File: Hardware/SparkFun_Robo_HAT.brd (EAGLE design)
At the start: 64.9 x 56.1 mm, 227 parts, among them J1 RASPBERRYPI-40-PIN-GPIO_PTH_R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, J11 EXT MTR PWR, J18 ISP, J2 CORTEX_DEBUGPTH, J20 USB C, J7 EXT SERVO PWR, J8 EXT 5V PWR, Q1 310mA/60V/1.6Ω, Q23 20V/0.2A/8MHz/1.2Ω/1Vth, Q24 20V/0.2A/8MHz/1.2Ω/1Vth, Q27 20V/0.2A/8MHz/1.2Ω/1Vth, Q28 20V/0.2A/8MHz/1.2Ω/1Vth, Q4 310mA/60V/1.6Ω, Q5 20V/4.2A/52mΩ/1.4W, Q7 20V/4.2A/52mΩ/1.4W, Q9 20V/4.2A/52mΩ/1.4W, U1 PCA9685, U4 ATTINY84-ARDUINO, U5 DRV8835, U6 CY8C4245LQI-483, U7 9DoF IMU, U8 1.8V/100mA

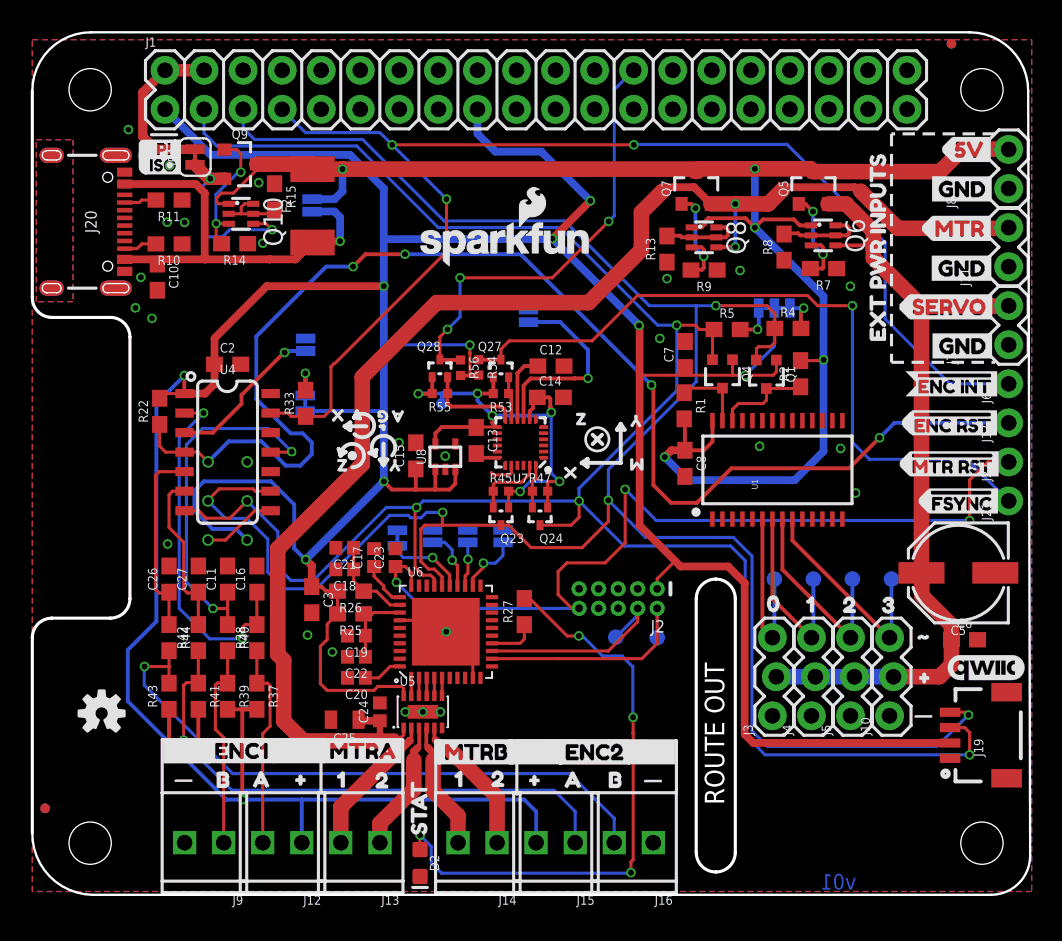
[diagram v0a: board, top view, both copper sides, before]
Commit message: sch cleanup and drc stuff in brd
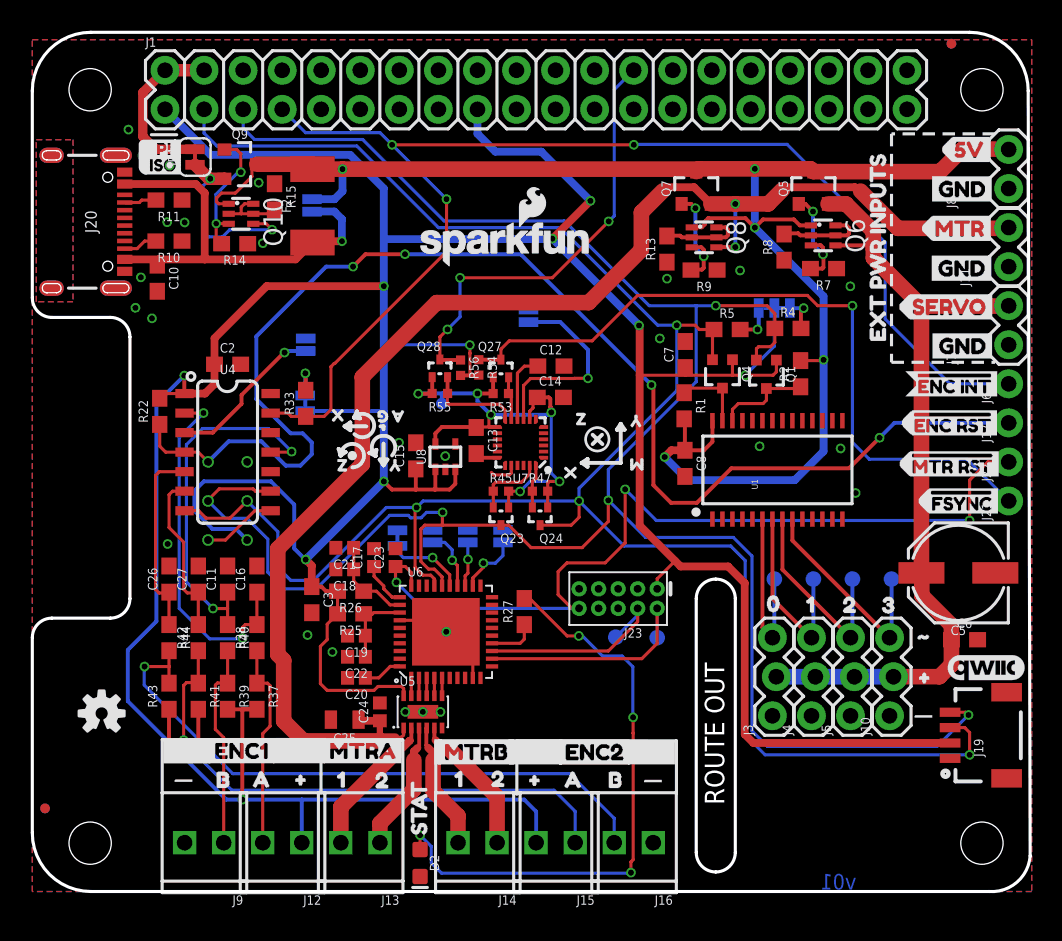
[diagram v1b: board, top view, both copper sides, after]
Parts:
- removed J2: CORTEX_DEBUGPTH, Pete_Connectors_Retired:2X5-PTH-1.27MM
- removed TP19: (no value), SparkFun-Connectors:TP_15TH
- added J23: CORTEX_JTAG_DEBUG_PTH, SparkFun-Connectors:2X5-PTH-1.27MM
- added TP9: (no value), SparkFun-Connectors:PAD.03X.03
- TP5: value 1.8V -> (none); device SparkFun-Connectors:PAD.03X.03 -> SparkFun-Connectors:TP_15TH
- moved TP5 41.2 mm to (61.0, 8.89), flipped to the top, turned to 270 degrees
- moved FRAME1 32.1 mm to (26.7, -20.3)
- moved R10 0.18 mm to (8.88, 42.3)
- moved C10 0.07 mm to (8.13, 39.9)
- renumbered TP11 to TP7, TP12 to TP8, TP18 to TP4, TP24 to TP6
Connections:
- net !MTR_RST: now also J23.10; no longer J2.10
- net 1.8V: now also TP9.P$1; no longer TP5.P$1
- net 3.3V: now also J23.1; no longer J2.1
- net GND: now also J23.3, J23.5, J23.7, J23.9; no longer J2.3, J2.5, J2.7, J2.9
- net P3.2: now also J23.2; no longer J2.2
- net P3.3: now also J23.4; no longer J2.4
- net SDA_3.3V: now also TP5.P$1; no longer TP19.P$1
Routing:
- net PI-5V: track 13.8 -> 13.1 mm
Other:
- board size 64.9 x 56.1 mm -> 64.9 x 55.9 mm
- board text added: "Servo Controller based on a design by Mike Hord Serial Controlled Motor Driver based on designs by Marshall Taylor, Alex Wende ICM-20948 based on a design by Owen Lyke ATTINY84 Encoder based on a design by Nathan Seidle"
- board text removed: "ATTiny84 Encoder based on a design by Nathan Seidle"
- board text removed: "ICM-20948 IMU based on a design by Owen Lyke"
- board text removed: "Serial Controlled Motor Driver based on a design by Marshall Taylor, Alex Wende"
- board text removed: "Servo Controller based on a design by Mike Hord"
